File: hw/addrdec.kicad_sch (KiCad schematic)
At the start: 5 parts, among them U10 74AS138, U11 74ACT00P, U5 74AHCT02, U7 74AS04N, U9 74AS27

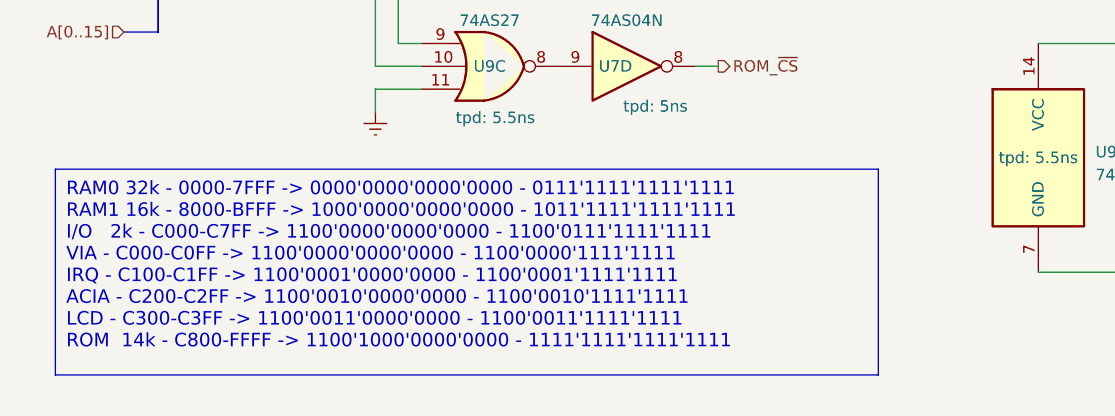
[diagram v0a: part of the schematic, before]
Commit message: clean up hw schematics
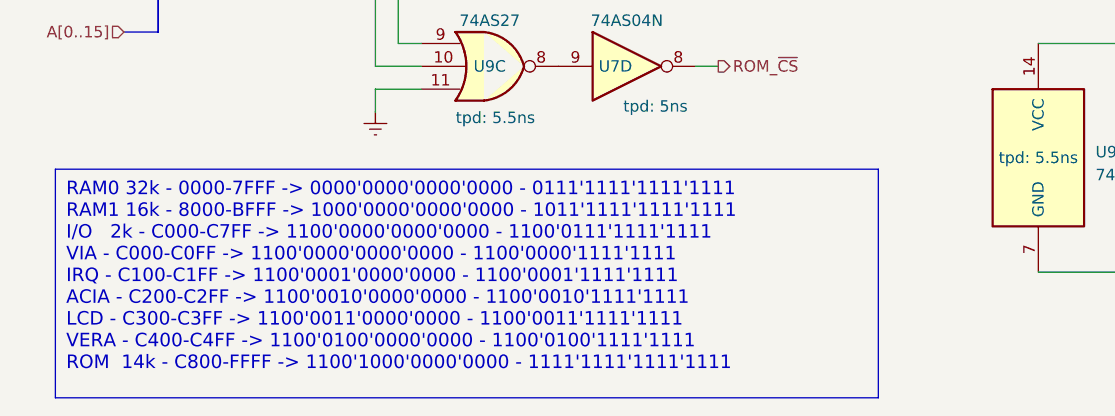
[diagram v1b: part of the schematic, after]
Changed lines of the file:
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@@
     (stroke (width 0) (type default))
   )
-  (text_box "RAM0 32k - 0000-7FFF -> 0000'0000'0000'0000 - 0111'1111'1111'1111\nRAM1 16k - 8000-BFFF -> 1000'0000'0000'0000 - 1011'1111'1111'1111\nI/O   2k - C000-C7FF -> 1100'0000'0000'0000 - 1100'0111'1111'1111\n     VIA - C000-C0FF -> 1100'0000'0000'0000 - 1100'0000'1111'1111\n     IRQ - C100-C1FF -> 1100'0001'0000'0000 - 1100'0001'1111'1111\n    ACIA - C200-C2FF -> 1100'0010'0000'0000 - 1100'0010'1111'1111\n     LCD - C300-C3FF -> 1100'0011'0000'0000 - 1100'0011'1111'1111\nROM  14k - C800-FFFF -> 1100'1000'0000'0000 - 1111'1111'1111'1111\n"
-    (at 16.51 114.3 0) (size 91.44 22.86)
+  (text_box "RAM0 32k - 0000-7FFF -> 0000'0000'0000'0000 - 0111'1111'1111'1111\nRAM1 16k - 8000-BFFF -> 1000'0000'0000'0000 - 1011'1111'1111'1111\nI/O   2k - C000-C7FF -> 1100'0000'0000'0000 - 1100'0111'1111'1111\n     VIA - C000-C0FF -> 1100'0000'0000'0000 - 1100'0000'1111'1111\n     IRQ - C100-C1FF -> 1100'0001'0000'0000 - 1100'0001'1111'1111\n    ACIA - C200-C2FF -> 1100'0010'0000'0000 - 1100'0010'1111'1111\n     LCD - C300-C3FF -> 1100'0011'0000'0000 - 1100'0011'1111'1111\n    VERA - C400-C4FF -> 1100'0100'0000'0000 - 1100'0100'1111'1111\nROM  14k - C800-FFFF -> 1100'1000'0000'0000 - 1111'1111'1111'1111\n"
+    (at 16.51 114.3 0) (size 91.44 25.4)
     (stroke (width 0) (type default))
     (fill (type none))
